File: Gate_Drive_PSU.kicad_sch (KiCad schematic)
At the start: 20 parts, among them U9 LM25184

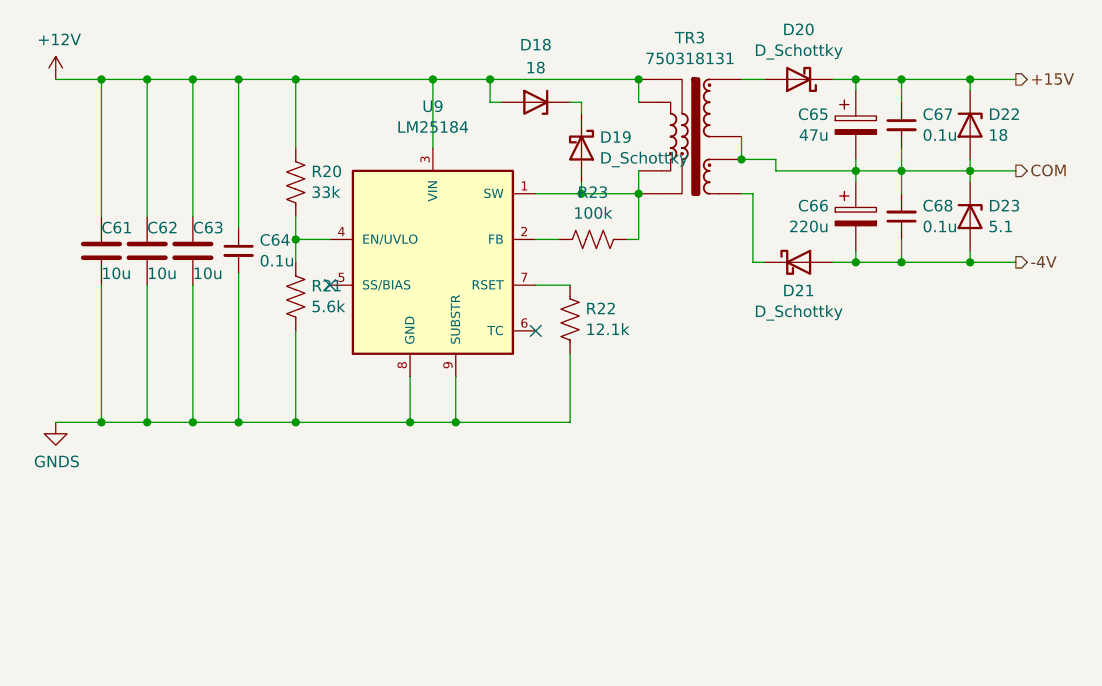
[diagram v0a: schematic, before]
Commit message: 1
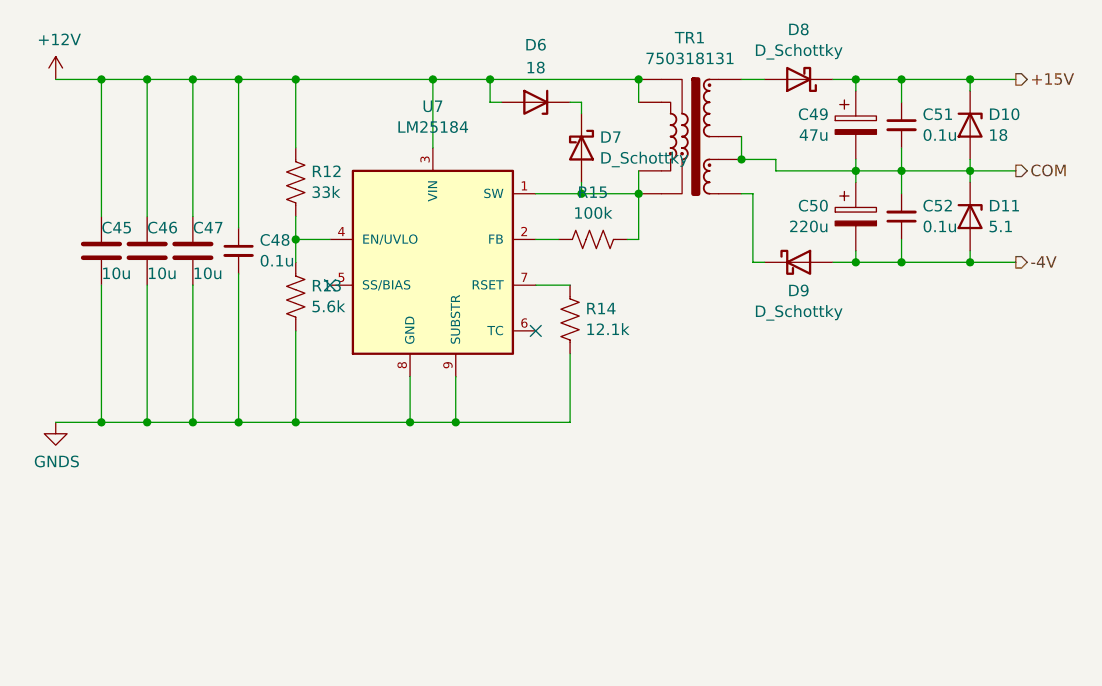
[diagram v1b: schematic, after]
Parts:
- renumbered C61 to C45, C62 to C46, C63 to C47, C64 to C48, C65 to C49, C66 to C50, C67 to C51, C68 to C52, D22 to D10, D23 to D11, D18 to D6, D19 to D7, D20 to D8, D21 to D9, R20 to R12, R21 to R13, R22 to R14, R23 to R15, TR3 to TR1, U9 to U7
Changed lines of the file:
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@@
   (symbol (lib_id "VFD:LM25184") (at 137.16 83.82 0)
     (in_bom yes) (on_board yes)
-    (property "Reference" "U9" (id 0) (at 137.16 66.5226 0))
+    (property "Reference" "U7" (id 0) (at 137.16 66.5226 0))
     (property "Value" "LM25184" (id 1) (at 137.16 68.834 0))
     (property "Footprint" "Package_SON:HVSON-8-1EP_4x4mm_P0.8mm_EP2.2x3.1mm" (id 2) (at 128.27 105.41 0)
@@
   (symbol (lib_id "Device:R_US") (at 154.94 81.28 270)
     (in_bom yes) (on_board yes)
-    (property "Reference" "R23" (id 0) (at 154.94 76.073 90))
+    (property "Reference" "R15" (id 0) (at 154.94 76.073 90))
     (property "Value" "100k" (id 1) (at 154.94 78.3844 90))
     (property "Footprint" "Resistor_SMD:R_0805_2012Metric" (id 2) (at 154.686 82.296 90)
@@
   (symbol (lib_id "Device:D_Schottky") (at 153.67 71.12 270)
     (in_bom yes) (on_board yes)
-    (property "Reference" "D19" (id 0) (at 155.702 69.9516 90)
+    (property "Reference" "D7" (id 0) (at 155.702 69.9516 90)
       (effects (font (size 1.27 1.27)) (justify left))
     )
@@
   (symbol (lib_id "Device:D_Zener") (at 148.59 66.04 180)
     (in_bom yes) (on_board yes)
-    (property "Reference" "D18" (id 0) (at 148.59 59.69 0))
+    (property "Reference" "D6" (id 0) (at 148.59 59.69 0))
     (property "Value" "18" (id 1) (at 148.59 62.23 0))
     (property "Footprint" "Diode_SMD:D_SMB" (id 2) (at 148.59 66.04 0)
@@
   (symbol (lib_id "Device:R_US") (at 152.4 90.17 0)
     (in_bom yes) (on_board yes)
-    (property "Reference" "R22" (id 0) (at 154.1272 89.0016 0)
+    (property "Reference" "R14" (id 0) (at 154.1272 89.0016 0)
       (effects (font (size 1.27 1.27)) (justify left))
     )
@@
   (symbol (lib_id "VFD:750318131") (at 166.37 69.85 0)
     (in_bom yes) (on_board yes)
-    (property "Reference" "TR3" (id 0) (at 165.735 58.9026 0))
+    (property "Reference" "TR1" (id 0) (at 165.735 58.9026 0))
     (property "Value" "750318131" (id 1) (at 165.735 61.214 0))
     (property "Footprint" "VFD:WE-AGDT_EP7" (id 2) (at 166.37 69.85 0)
@@
   (symbol (lib_id "Device:C") (at 110.49 82.55 0)
     (in_bom yes) (on_board yes)
-    (property "Reference" "C63" (id 0) (at 110.49 80.01 0)
+    (property "Reference" "C47" (id 0) (at 110.49 80.01 0)
       (effects (font (size 1.27 1.27)) (justify left))
     )
@@
   (symbol (lib_id "Device:C") (at 105.41 82.55 0)
     (in_bom yes) (on_board yes)
-    (property "Reference" "C62" (id 0) (at 105.41 80.01 0)
+    (property "Reference" "C46" (id 0) (at 105.41 80.01 0)
       (effects (font (size 1.27 1.27)) (justify left))
     )
@@
   (symbol (lib_id "Device:C") (at 100.33 82.55 0)
     (in_bom yes) (on_board yes)
-    (property "Reference" "C61" (id 0) (at 100.33 80.01 0)
+    (property "Reference" "C45" (id 0) (at 100.33 80.01 0)
       (effects (font (size 1.27 1.27)) (justify left))
     )
@@
   (symbol (lib_id "Device:C_Small") (at 115.57 82.55 0)
     (in_bom yes) (on_board yes)
-    (property "Reference" "C64" (id 0) (at 117.9068 81.3816 0)
+    (property "Reference" "C48" (id 0) (at 117.9068 81.3816 0)
       (effects (font (size 1.27 1.27)) (justify left))
     )
@@
   (symbol (lib_id "Device:R_US") (at 121.92 74.93 0)
     (in_bom yes) (on_board yes)
-    (property "Reference" "R20" (id 0) (at 123.6472 73.7616 0)
+    (property "Reference" "R12" (id 0) (at 123.6472 73.7616 0)
       (effects (font (size 1.27 1.27)) (justify left))
     )
@@
   (symbol (lib_id "Device:R_US") (at 121.92 87.63 0)
     (in_bom yes) (on_board yes)
-    (property "Reference" "R21" (id 0) (at 123.6472 86.4616 0)
+    (property "Reference" "R13" (id 0) (at 123.6472 86.4616 0)
       (effects (font (size 1.27 1.27)) (justify left))
     )
@@
   (symbol (lib_id "Device:C_Polarized") (at 184.15 68.58 0)
     (in_bom yes) (on_board yes)
-    (property "Reference" "C65" (id 0) (at 181.1528 67.4116 0)
+    (property "Reference" "C49" (id 0) (at 181.1528 67.4116 0)
       (effects (font (size 1.27 1.27)) (justify right))
     )
@@
   (symbol (lib_id "Device:C_Polarized") (at 184.15 78.74 0)
     (in_bom yes) (on_board yes)
-    (property "Reference" "C66" (id 0) (at 181.1528 77.5716 0)
+    (property "Reference" "C50" (id 0) (at 181.1528 77.5716 0)
       (effects (font (size 1.27 1.27)) (justify right))
     )
@@
   (symbol (lib_id "Device:D_Schottky") (at 177.8 63.5 180)
     (in_bom yes) (on_board yes)
-    (property "Reference" "D20" (id 0) (at 177.8 57.9882 0))
+    (property "Reference" "D8" (id 0) (at 177.8 57.9882 0))
     (property "Value" "D_Schottky" (id 1) (at 177.8 60.2996 0))
     (property "Footprint" "Diode_SMD:D_SOD-128" (id 2) (at 177.8 63.5 0)
@@
   (symbol (lib_id "Device:D_Schottky") (at 177.8 83.82 0)
     (in_bom yes) (on_board yes)
-    (property "Reference" "D21" (id 0) (at 177.8 86.995 0))
+    (property "Reference" "D9" (id 0) (at 177.8 86.995 0))
     (property "Value" "D_Schottky" (id 1) (at 177.8 89.3064 0))
     (property "Footprint" "Diode_SMD:D_SOD-128" (id 2) (at 177.8 83.82 0)
@@
   (symbol (lib_id "Device:D_Zener") (at 196.85 68.58 270)
     (in_bom yes) (on_board yes)
-    (property "Reference" "D22" (id 0) (at 198.882 67.4116 90)
+    (property "Reference" "D10" (id 0) (at 198.882 67.4116 90)
       (effects (font (size 1.27 1.27)) (justify left))
     )
@@
   (symbol (lib_id "Device:D_Zener") (at 196.85 78.74 270)
     (in_bom yes) (on_board yes)
-    (property "Reference" "D23" (id 0) (at 198.882 77.5716 90)
+    (property "Reference" "D11" (id 0) (at 198.882 77.5716 90)
       (effects (font (size 1.27 1.27)) (justify left))
     )
@@
   (symbol (lib_id "Device:C_Small") (at 189.23 68.58 0)
     (in_bom yes) (on_board yes)
-    (property "Reference" "C67" (id 0) (at 191.5668 67.4116 0)
+    (property "Reference" "C51" (id 0) (at 191.5668 67.4116 0)
       (effects (font (size 1.27 1.27)) (justify left))
     )
@@
   (symbol (lib_id "Device:C_Small") (at 189.23 78.74 180)
     (in_bom yes) (on_board yes)
-    (property "Reference" "C68" (id 0) (at 191.5668 77.5716 0)
+    (property "Reference" "C52" (id 0) (at 191.5668 77.5716 0)
       (effects (font (size 1.27 1.27)) (justify right))
     )
@@
   (symbol (lib_id "power:+12V") (at 95.25 63.5 0)
     (in_bom yes) (on_board yes)
-    (property "Reference" "#PWR026" (id 0) (at 95.25 67.31 0)
+    (property "Reference" "#PWR022" (id 0) (at 95.25 67.31 0)
       (effects (font (size 1.27 1.27)) hide)
     )
@@
   (symbol (lib_id "power:GNDS") (at 95.25 101.6 0)
     (in_bom yes) (on_board yes)
-    (property "Reference" "#PWR027" (id 0) (at 95.25 107.95 0)
-      (effects (font (size 1.27 1.27)) hide)
-    )
+    (property "Reference" "#PWR023" (id 0) (at 95.25 107.95 0)
+      (effects (font (size 1.27 1.27)) hide)
+    )

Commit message: 1
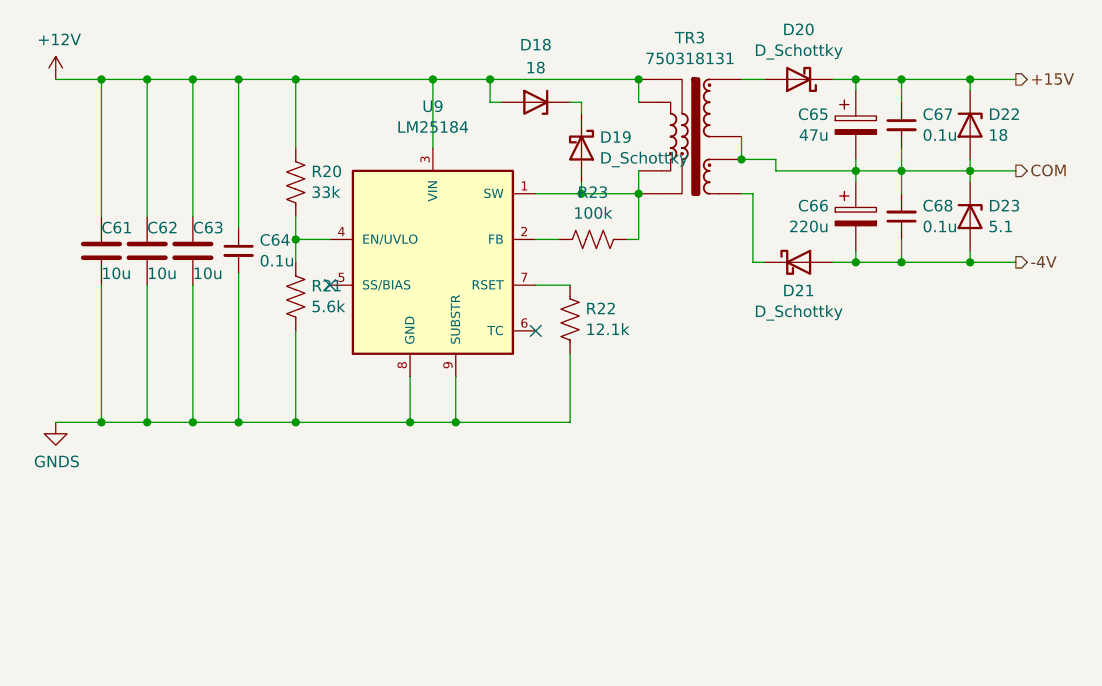
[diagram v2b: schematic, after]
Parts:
- renumbered C45 to C61, C46 to C62, C47 to C63, C48 to C64, C49 to C65, C50 to C66, C51 to C67, C52 to C68, D6 to D18, D7 to D19, D8 to D20, D9 to D21, D10 to D22, D11 to D23, R12 to R20, R13 to R21, R14 to R22, R15 to R23, TR1 to TR3, U7 to U9
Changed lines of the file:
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@@
     (effects (font (size 1.27 1.27)) (justify left))
   )
-  (symbol (lib_id "VFD:LM25184") (at 137.16 83.82 0)
-    (in_bom yes) (on_board yes)
-    (property "Reference" "U7" (id 0) (at 137.16 66.5226 0))
+  (symbol (lib_id "VFD:LM25184") (at 137.16 83.82 0) (unit 1)
+    (in_bom yes) (on_board yes)
+    (property "Reference" "U9" (id 0) (at 137.16 66.5226 0))
     (property "Value" "LM25184" (id 1) (at 137.16 68.834 0))
     (property "Footprint" "Package_SON:HVSON-8-1EP_4x4mm_P0.8mm_EP2.2x3.1mm" (id 2) (at 128.27 105.41 0)
@@
     (pin "9")
   )
-  (symbol (lib_id "Device:R_US") (at 154.94 81.28 270)
-    (in_bom yes) (on_board yes)
-    (property "Reference" "R15" (id 0) (at 154.94 76.073 90))
+  (symbol (lib_id "Device:R_US") (at 154.94 81.28 270) (unit 1)
+    (in_bom yes) (on_board yes)
+    (property "Reference" "R23" (id 0) (at 154.94 76.073 90))
     (property "Value" "100k" (id 1) (at 154.94 78.3844 90))
     (property "Footprint" "Resistor_SMD:R_0805_2012Metric" (id 2) (at 154.686 82.296 90)
@@
     (pin "2")
   )
-  (symbol (lib_id "Device:D_Schottky") (at 153.67 71.12 270)
-    (in_bom yes) (on_board yes)
-    (property "Reference" "D7" (id 0) (at 155.702 69.9516 90)
+  (symbol (lib_id "Device:D_Schottky") (at 153.67 71.12 270) (unit 1)
+    (in_bom yes) (on_board yes)
+    (property "Reference" "D19" (id 0) (at 155.702 69.9516 90)
       (effects (font (size 1.27 1.27)) (justify left))
     )
@@
     (pin "2")
   )
-  (symbol (lib_id "Device:D_Zener") (at 148.59 66.04 180)
-    (in_bom yes) (on_board yes)
-    (property "Reference" "D6" (id 0) (at 148.59 59.69 0))
+  (symbol (lib_id "Device:D_Zener") (at 148.59 66.04 180) (unit 1)
+    (in_bom yes) (on_board yes)
+    (property "Reference" "D18" (id 0) (at 148.59 59.69 0))
     (property "Value" "18" (id 1) (at 148.59 62.23 0))
     (property "Footprint" "Diode_SMD:D_SMB" (id 2) (at 148.59 66.04 0)
@@
     (pin "2")
   )
-  (symbol (lib_id "Device:R_US") (at 152.4 90.17 0)
-    (in_bom yes) (on_board yes)
-    (property "Reference" "R14" (id 0) (at 154.1272 89.0016 0)
+  (symbol (lib_id "Device:R_US") (at 152.4 90.17 0) (unit 1)
+    (in_bom yes) (on_board yes)
+    (property "Reference" "R22" (id 0) (at 154.1272 89.0016 0)
       (effects (font (size 1.27 1.27)) (justify left))
     )
@@
     (pin "2")
   )
-  (symbol (lib_id "VFD:750318131") (at 166.37 69.85 0)
-    (in_bom yes) (on_board yes)
-    (property "Reference" "TR1" (id 0) (at 165.735 58.9026 0))
+  (symbol (lib_id "VFD:750318131") (at 166.37 69.85 0) (unit 1)
+    (in_bom yes) (on_board yes)
+    (property "Reference" "TR3" (id 0) (at 165.735 58.9026 0))
     (property "Value" "750318131" (id 1) (at 165.735 61.214 0))
     (property "Footprint" "VFD:WE-AGDT_EP7" (id 2) (at 166.37 69.85 0)
@@
     (pin "8")
   )
-  (symbol (lib_id "Device:C") (at 110.49 82.55 0)
-    (in_bom yes) (on_board yes)
-    (property "Reference" "C47" (id 0) (at 110.49 80.01 0)
+  (symbol (lib_id "Device:C") (at 110.49 82.55 0) (unit 1)
+    (in_bom yes) (on_board yes)
+    (property "Reference" "C63" (id 0) (at 110.49 80.01 0)
       (effects (font (size 1.27 1.27)) (justify left))
     )
@@
     (pin "2")
   )
-  (symbol (lib_id "Device:C") (at 105.41 82.55 0)
-    (in_bom yes) (on_board yes)
-    (property "Reference" "C46" (id 0) (at 105.41 80.01 0)
+  (symbol (lib_id "Device:C") (at 105.41 82.55 0) (unit 1)
+    (in_bom yes) (on_board yes)
+    (property "Reference" "C62" (id 0) (at 105.41 80.01 0)
       (effects (font (size 1.27 1.27)) (justify left))
     )
@@
     (pin "2")
   )
-  (symbol (lib_id "Device:C") (at 100.33 82.55 0)
-    (in_bom yes) (on_board yes)
-    (property "Reference" "C45" (id 0) (at 100.33 80.01 0)
+  (symbol (lib_id "Device:C") (at 100.33 82.55 0) (unit 1)
+    (in_bom yes) (on_board yes)
+    (property "Reference" "C61" (id 0) (at 100.33 80.01 0)
       (effects (font (size 1.27 1.27)) (justify left))
     )
@@
     (pin "2")
   )
-  (symbol (lib_id "Device:C_Small") (at 115.57 82.55 0)
-    (in_bom yes) (on_board yes)
-    (property "Reference" "C48" (id 0) (at 117.9068 81.3816 0)
+  (symbol (lib_id "Device:C_Small") (at 115.57 82.55 0) (unit 1)
+    (in_bom yes) (on_board yes)
+    (property "Reference" "C64" (id 0) (at 117.9068 81.3816 0)
       (effects (font (size 1.27 1.27)) (justify left))
     )
@@
     (pin "2")
   )
-  (symbol (lib_id "Device:R_US") (at 121.92 74.93 0)
-    (in_bom yes) (on_board yes)
-    (property "Reference" "R12" (id 0) (at 123.6472 73.7616 0)
+  (symbol (lib_id "Device:R_US") (at 121.92 74.93 0) (unit 1)
+    (in_bom yes) (on_board yes)
+    (property "Reference" "R20" (id 0) (at 123.6472 73.7616 0)
       (effects (font (size 1.27 1.27)) (justify left))
     )
@@
     (pin "2")
   )
-  (symbol (lib_id "Device:R_US") (at 121.92 87.63 0)
-    (in_bom yes) (on_board yes)
-    (property "Reference" "R13" (id 0) (at 123.6472 86.4616 0)
+  (symbol (lib_id "Device:R_US") (at 121.92 87.63 0) (unit 1)
+    (in_bom yes) (on_board yes)
+    (property "Reference" "R21" (id 0) (at 123.6472 86.4616 0)
       (effects (font (size 1.27 1.27)) (justify left))
     )
@@
     (pin "2")
   )
-  (symbol (lib_id "Device:C_Polarized") (at 184.15 68.58 0)
-    (in_bom yes) (on_board yes)
-    (property "Reference" "C49" (id 0) (at 181.1528 67.4116 0)
+  (symbol (lib_id "Device:C_Polarized") (at 184.15 68.58 0) (unit 1)
+    (in_bom yes) (on_board yes)
+    (property "Reference" "C65" (id 0) (at 181.1528 67.4116 0)
       (effects (font (size 1.27 1.27)) (justify right))
     )
@@
     (pin "2")
   )
-  (symbol (lib_id "Device:C_Polarized") (at 184.15 78.74 0)
-    (in_bom yes) (on_board yes)
-    (property "Reference" "C50" (id 0) (at 181.1528 77.5716 0)
+  (symbol (lib_id "Device:C_Polarized") (at 184.15 78.74 0) (unit 1)
+    (in_bom yes) (on_board yes)
+    (property "Reference" "C66" (id 0) (at 181.1528 77.5716 0)
       (effects (font (size 1.27 1.27)) (justify right))
     )
@@
     (pin "2")
   )
-  (symbol (lib_id "Device:D_Schottky") (at 177.8 63.5 180)
-    (in_bom yes) (on_board yes)
-    (property "Reference" "D8" (id 0) (at 177.8 57.9882 0))
+  (symbol (lib_id "Device:D_Schottky") (at 177.8 63.5 180) (unit 1)
+    (in_bom yes) (on_board yes)
+    (property "Reference" "D20" (id 0) (at 177.8 57.9882 0))
     (property "Value" "D_Schottky" (id 1) (at 177.8 60.2996 0))
     (property "Footprint" "Diode_SMD:D_SOD-128" (id 2) (at 177.8 63.5 0)
@@
     (pin "2")
   )
-  (symbol (lib_id "Device:D_Schottky") (at 177.8 83.82 0)
-    (in_bom yes) (on_board yes)
-    (property "Reference" "D9" (id 0) (at 177.8 86.995 0))
+  (symbol (lib_id "Device:D_Schottky") (at 177.8 83.82 0) (unit 1)
+    (in_bom yes) (on_board yes)
+    (property "Reference" "D21" (id 0) (at 177.8 86.995 0))
     (property "Value" "D_Schottky" (id 1) (at 177.8 89.3064 0))
     (property "Footprint" "Diode_SMD:D_SOD-128" (id 2) (at 177.8 83.82 0)
@@
     (pin "2")
   )
-  (symbol (lib_id "Device:D_Zener") (at 196.85 68.58 270)
-    (in_bom yes) (on_board yes)
-    (property "Reference" "D10" (id 0) (at 198.882 67.4116 90)
+  (symbol (lib_id "Device:D_Zener") (at 196.85 68.58 270) (unit 1)
+    (in_bom yes) (on_board yes)
+    (property "Reference" "D22" (id 0) (at 198.882 67.4116 90)
       (effects (font (size 1.27 1.27)) (justify left))
     )
@@
     (pin "2")
   )
-  (symbol (lib_id "Device:D_Zener") (at 196.85 78.74 270)
-    (in_bom yes) (on_board yes)
-    (property "Reference" "D11" (id 0) (at 198.882 77.5716 90)
+  (symbol (lib_id "Device:D_Zener") (at 196.85 78.74 270) (unit 1)
+    (in_bom yes) (on_board yes)
+    (property "Reference" "D23" (id 0) (at 198.882 77.5716 90)
       (effects (font (size 1.27 1.27)) (justify left))
     )
@@
     (pin "2")
   )
-  (symbol (lib_id "Device:C_Small") (at 189.23 68.58 0)
-    (in_bom yes) (on_board yes)
-    (property "Reference" "C51" (id 0) (at 191.5668 67.4116 0)
+  (symbol (lib_id "Device:C_Small") (at 189.23 68.58 0) (unit 1)
+    (in_bom yes) (on_board yes)
+    (property "Reference" "C67" (id 0) (at 191.5668 67.4116 0)
       (effects (font (size 1.27 1.27)) (justify left))
     )
@@
     (pin "2")
   )
-  (symbol (lib_id "Device:C_Small") (at 189.23 78.74 180)
-    (in_bom yes) (on_board yes)
-    (property "Reference" "C52" (id 0) (at 191.5668 77.5716 0)
+  (symbol (lib_id "Device:C_Small") (at 189.23 78.74 180) (unit 1)
+    (in_bom yes) (on_board yes)
+    (property "Reference" "C68" (id 0) (at 191.5668 77.5716 0)
       (effects (font (size 1.27 1.27)) (justify right))
     )
@@
     (pin "2")
   )
-  (symbol (lib_id "power:+12V") (at 95.25 63.5 0)
-    (in_bom yes) (on_board yes)
-    (property "Reference" "#PWR022" (id 0) (at 95.25 67.31 0)
+  (symbol (lib_id "power:+12V") (at 95.25 63.5 0) (unit 1)
+    (in_bom yes) (on_board yes)
+    (property "Reference" "#PWR026" (id 0) (at 95.25 67.31 0)
       (effects (font (size 1.27 1.27)) hide)
     )
@@
     (pin "1")
   )
-  (symbol (lib_id "power:GNDS") (at 95.25 101.6 0)
-    (in_bom yes) (on_board yes)
-    (property "Reference" "#PWR023" (id 0) (at 95.25 107.95 0)
-      (effects (font (size 1.27 1.27)) hide)
-    )
+  (symbol (lib_id "power:GNDS") (at 95.25 101.6 0) (unit 1)
+    (in_bom yes) (on_board yes)
+    (property "Reference" "#PWR027" (id 0) (at 95.25 107.95 0)
+      (effects (font (size 1.27 1.27)) hide)
+    )

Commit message: 1
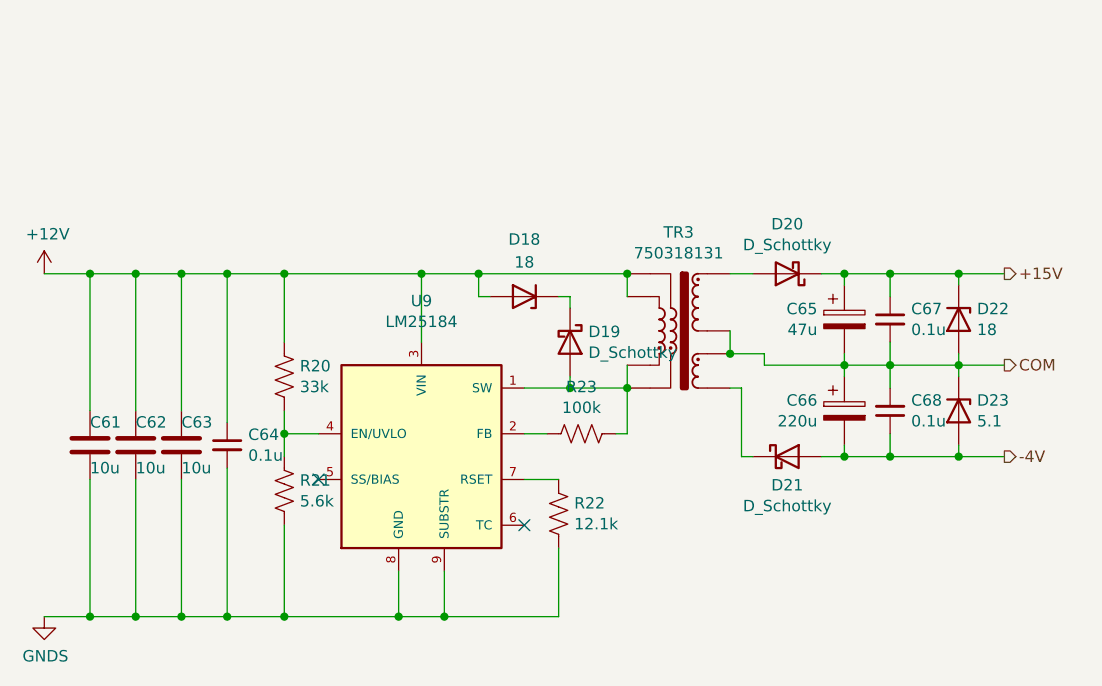
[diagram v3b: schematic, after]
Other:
- moved on the sheet: C61, C62, C63, C64, C65, C66, C67, C68, D18, D19, D20, D21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
